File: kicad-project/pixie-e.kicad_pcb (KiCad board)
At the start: 2 copper layers, 55 x 50 mm, 54 parts, among them J1 PWR, J2 ANT, J3 SP, J4 KEY, Q1 2N2222, Q2 2N2222, Q3 2N2222, Q4 2N3906, Q5 2N7000, SW1 PWR, SW2 SW, U1 LM386, U2 STC15W104, U3 LM78L05_TO92, Y1 7.023MHz

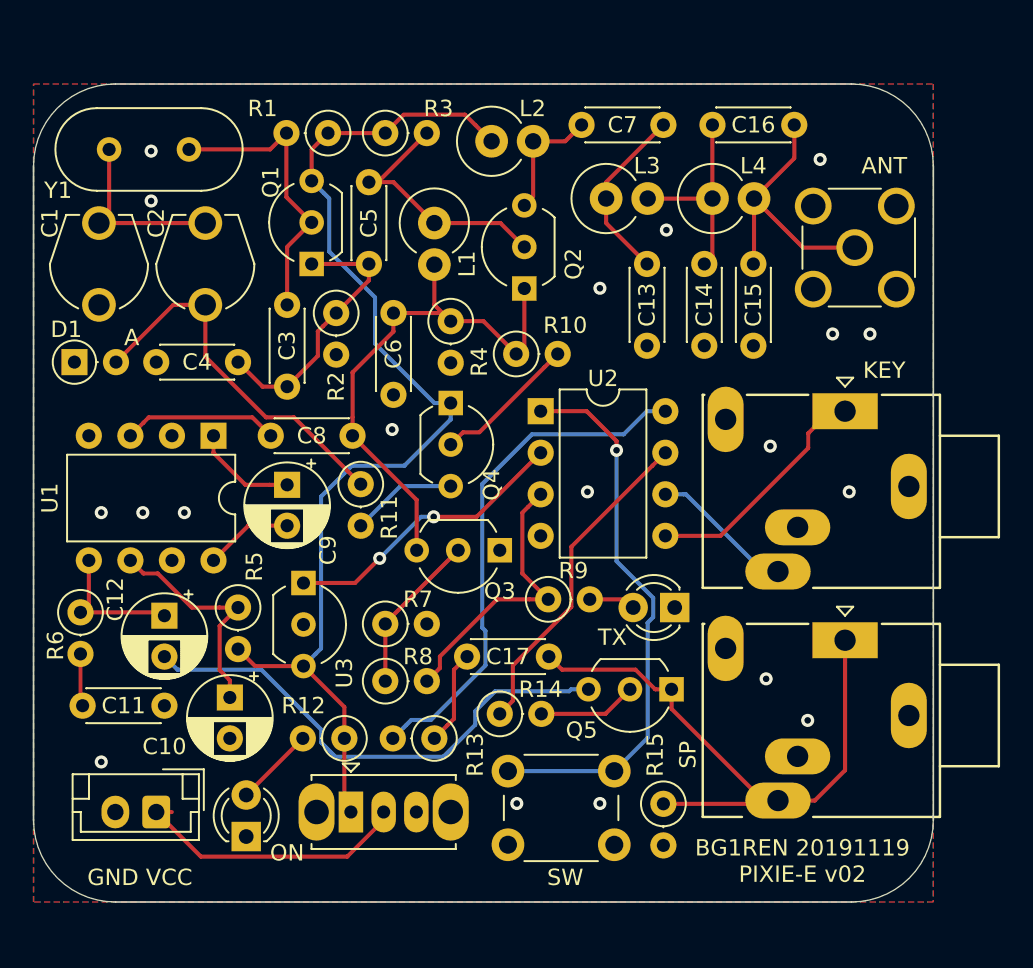
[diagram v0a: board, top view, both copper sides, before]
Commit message: Finish the 1st smt version.
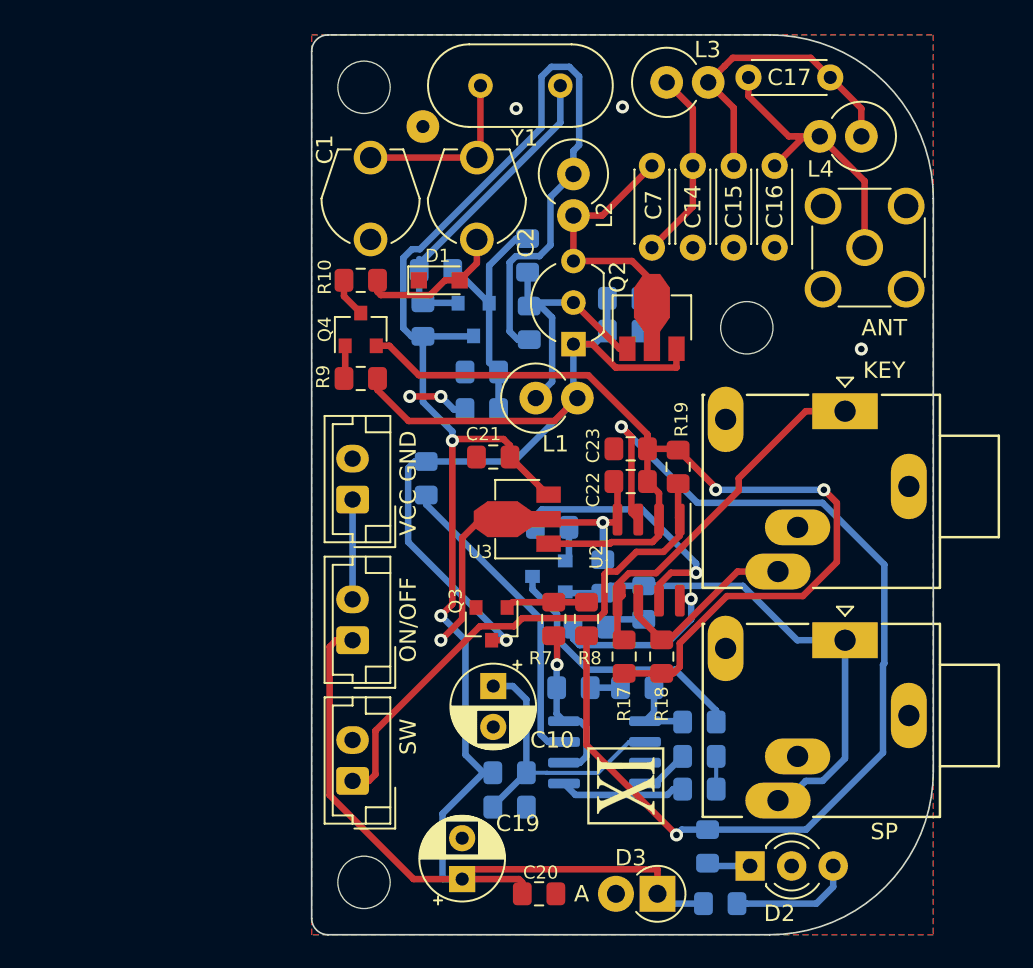
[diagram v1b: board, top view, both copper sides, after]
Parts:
- added C11: 100n, Capacitor_SMD:C_0805_2012Metric_Pad1.15x1.40mm_HandSolder, B.Cu at (129.1, 94.2)
- added C19: 100u, Capacitor_THT:CP_Radial_D5.0mm_P2.50mm, F.Cu at (126.2, 98.6)
- added C20: 100n, Capacitor_SMD:C_0805_2012Metric_Pad1.15x1.40mm_HandSolder, F.Cu at (130.9, 99.5)
- added C21: 330n, Capacitor_SMD:C_0805_2012Metric_Pad1.15x1.40mm_HandSolder, F.Cu at (128.1, 72.8)
- added C22: 100n, Capacitor_SMD:C_0805_2012Metric_Pad1.15x1.40mm_HandSolder, F.Cu at (136.5, 74.3)
- added C23: 10u, Capacitor_SMD:C_0805_2012Metric_Pad1.15x1.40mm_HandSolder, F.Cu at (136.5, 72.3)
- added G***: LOGO, xi:xi-logo-a-07_07, B.Cu at (124.3, 79.6)
- added G***: LOGO, xi:xi-logo-c-05_05, F.Cu at (136.2, 92.9)
- added R16: 1K, Resistor_SMD:R_0805_2012Metric_Pad1.15x1.40mm_HandSolder, B.Cu at (140.7, 93.1)
- added R17: 10K, Resistor_SMD:R_0805_2012Metric_Pad1.15x1.40mm_HandSolder, F.Cu at (136.1, 85.0)
- added R18: 10K, Resistor_SMD:R_0805_2012Metric_Pad1.15x1.40mm_HandSolder, F.Cu at (138.4, 85.0)
- added R19: 10K, Resistor_SMD:R_0805_2012Metric_Pad1.15x1.40mm_HandSolder, F.Cu at (139.4, 73.4)
- added REF**: SOT-89-3, Package_TO_SOT_SMD:SOT-89-3, F.Cu at (137.8, 64.7)
- added REF**: FreeSolderWirePad_1x01_Drill0.8mm, bg1ren:FreeSolderWirePad_1x01_Drill0.8mm, F.Cu at (123.8, 52.6)
- added REF**: MountingHole_3.2mm_M3_DIN965, MountingHole:MountingHole_3.2mm_M3_DIN965, F.Cu at (120.2, 98.8)
- added REF**: MountingHole_3.2mm_M3_DIN965, MountingHole:MountingHole_3.2mm_M3_DIN965, F.Cu at (120.2, 50.2)
- added REF**: MountingHole_3.2mm_M3_DIN965, MountingHole:MountingHole_3.2mm_M3_DIN965, F.Cu at (143.6, 64.9)
- C12: renamed from C11; footprint Capacitor_THT:C_Disc_D4.3mm_W1.9mm_P5.00mm -> Capacitor_SMD:C_0805_2012Metric_Pad1.15x1.40mm_HandSolder; moved to B.Cu
- C13: renamed from C12; footprint Capacitor_THT:CP_Radial_D5.0mm_P2.50mm -> Capacitor_SMD:C_0805_2012Metric_Pad1.15x1.40mm_HandSolder; moved to B.Cu
- C18: renamed from C17; footprint Capacitor_THT:C_Disc_D4.3mm_W1.9mm_P5.00mm -> Capacitor_SMD:C_0805_2012Metric_Pad1.15x1.40mm_HandSolder; moved to B.Cu
- C3, C4, C5, C6, C8: footprint Capacitor_THT:C_Disc_D4.3mm_W1.9mm_P5.00mm -> Capacitor_SMD:C_0805_2012Metric_Pad1.15x1.40mm_HandSolder; moved to B.Cu
- C7: value 10n -> 100n
- C9: footprint Capacitor_THT:CP_Radial_D5.0mm_P2.50mm -> Capacitor_SMD:C_0805_2012Metric_Pad1.15x1.40mm_HandSolder; moved to B.Cu
- D1: footprint Diode_THT:D_DO-35_SOD27_P2.54mm_Vertical_AnodeUp -> Diode_SMD:D_SOD-323_HandSoldering
- D2: value RED -> LED_Dual_ACA; footprint LED_THT:LED_D3.0mm -> LED_THT:LED_D3.0mm-3
- D3: value YELLO -> 1N4001; footprint LED_THT:LED_D3.0mm -> Diode_THT:D_DO-41_SOD81_P2.54mm_Vertical_AnodeUp
- Q1: footprint Package_TO_SOT_THT:TO-92_Inline_Wide -> Package_TO_SOT_SMD:SOT-23; moved to B.Cu
- Q3, Q4: footprint Package_TO_SOT_THT:TO-92_Inline_Wide -> Package_TO_SOT_SMD:SOT-23
- Q5: value 2N7000 -> 2N7002; footprint Package_TO_SOT_THT:TO-92_Inline_Wide -> Package_TO_SOT_SMD:SOT-23; moved to B.Cu
- R1, R13, R14, R15, R3, R4, R6: footprint Resistor_THT:R_Axial_DIN0207_L6.3mm_D2.5mm_P2.54mm_Vertical -> Resistor_SMD:R_0805_2012Metric_Pad1.15x1.40mm_HandSolder; moved to B.Cu
- R10: renamed from R11; value 4.7K -> 1K; footprint Resistor_THT:R_Axial_DIN0207_L6.3mm_D2.5mm_P2.54mm_Vertical -> Resistor_SMD:R_0805_2012Metric_Pad1.15x1.40mm_HandSolder
- R11: renamed from R12; footprint Resistor_THT:R_Axial_DIN0207_L6.3mm_D2.5mm_P2.54mm_Vertical -> Resistor_SMD:R_0805_2012Metric_Pad1.15x1.40mm_HandSolder; moved to B.Cu
- R12: renamed from R9; footprint Resistor_THT:R_Axial_DIN0207_L6.3mm_D2.5mm_P2.54mm_Vertical -> Resistor_SMD:R_0805_2012Metric_Pad1.15x1.40mm_HandSolder; moved to B.Cu
- R2: value 470 -> 1K; footprint Resistor_THT:R_Axial_DIN0207_L6.3mm_D2.5mm_P2.54mm_Vertical -> Resistor_SMD:R_0805_2012Metric_Pad1.15x1.40mm_HandSolder; moved to B.Cu
- R5: value 1K -> 10; footprint Resistor_THT:R_Axial_DIN0207_L6.3mm_D2.5mm_P2.54mm_Vertical -> Resistor_SMD:R_0805_2012Metric_Pad1.15x1.40mm_HandSolder; moved to B.Cu
- R7, R8: footprint Resistor_THT:R_Axial_DIN0207_L6.3mm_D2.5mm_P2.54mm_Vertical -> Resistor_SMD:R_0805_2012Metric_Pad1.15x1.40mm_HandSolder
- R9: renamed from R10; footprint Resistor_THT:R_Axial_DIN0207_L6.3mm_D2.5mm_P2.54mm_Vertical -> Resistor_SMD:R_0805_2012Metric_Pad1.15x1.40mm_HandSolder
- SW1: value PWR -> ON/OFF; footprint Button_Switch_THT:SW_Slide_1P2T_CK_OS102011MS2Q -> Connector_JST:JST_EH_B2B-EH-A_1x02_P2.50mm_Vertical
- SW2: footprint Button_Switch_THT:SW_PUSH_6mm -> Connector_JST:JST_EH_B2B-EH-A_1x02_P2.50mm_Vertical
- U1: footprint Package_DIP:DIP-8_W7.62mm -> Package_SO:SOIC-8_3.9x4.9mm_P1.27mm; moved to B.Cu
- U2: footprint Package_DIP:DIP-8_W7.62mm -> Package_SO:SOIC-8_3.9x4.9mm_P1.27mm
- U3: footprint Package_TO_SOT_THT:TO-92_Inline_Wide -> Package_TO_SOT_SMD:SOT-89-3
- Y1: footprint Crystal:Crystal_HC49-4H_Vertical -> Crystal:Crystal_HC49-U_Vertical
- moved R6 34.3 mm to (136.9, 86.9), turned to 180 degrees
- moved C13 33.3 mm to (140.7, 89.0), turned to 0 degrees
- moved U1 30.8 mm to (134.9, 90.8), turned to 0 degrees
- moved C9 30.2 mm to (140.7, 91.1), turned to 180 degrees
- moved D3 25.4 mm to (138.1, 99.5), turned to 180 degrees
- moved R11 25.1 mm to (142.0, 100.1)
- moved C12 25.0 mm to (133.0, 86.9), turned to 0 degrees
- moved Y1 23.0 mm to (132.2, 50.1)
- moved D1 22.9 mm to (124.8, 62.0)
- moved J1 22.6 mm to (119.5, 75.4), turned to 90 degrees
- moved R5 19.4 mm to (129.1, 92.1), turned to 180 degrees
- moved R12 18.0 mm to (141.2, 96.6), turned to 270 degrees
- moved C1 17.1 mm to (120.6, 57.0)
- moved C2 17.1 mm to (127.1, 57.0)
- moved D2 16.5 mm to (143.8, 97.8), turned to 0 degrees
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- renumbered C13 to C14, C14 to C15, C15 to C16, C16 to C17
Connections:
- net Net-(R8-Pad2) renamed TX-LED
- D2 pad 1: GND -> Net-(D2-Pad1)
- D2 pad 2: Net-(D2-Pad2) -> GND
- D3 pad 1: GND -> VCC
- D3 pad 2: Net-(D3-Pad2) -> GND
- Q1 pad 1: Net-(C3-Pad2) -> Net-(C3-Pad1)
- Q1 pad 2: Net-(C3-Pad1) -> Net-(C3-Pad2)
- Q3 pad 1: GND -> Net-(Q3-Pad1)
- Q3 pad 2: Net-(Q3-Pad2) -> GND
- Q4 pad 1: VCC -> Net-(Q4-Pad1)
- Q4 pad 2: Net-(Q4-Pad2) -> 5V
- Q5 pad 1: Phone -> Net-(Q5-Pad1)
- Q5 pad 2: Net-(Q5-Pad2) -> Phone
- R11 pad 1: VCC -> Net-(D2-Pad3)
- R11 pad 2: Net-(D3-Pad2) -> VCC
- R12 pad 2: Net-(D2-Pad2) -> Net-(D2-Pad1)
- R14 pad 2: Net-(Q5-Pad2) -> Net-(Q5-Pad1)
- R7 pad 1: Net-(Q3-Pad2) -> Net-(Q3-Pad1)
- R8 pad 1: Net-(Q3-Pad2) -> Net-(Q3-Pad1)
- R9 pad 2: Net-(Q4-Pad2) -> Net-(Q4-Pad1)
- U1 pad 1: Net-(C9-Pad1) -> Net-(R16-Pad2)
- U1 pad 7: Net-(U1-Pad7) -> (no net)
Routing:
- net VCC: track 68.4 -> 134.9 mm, vias 0 -> 2
- net TX-LED: track 17.4 -> 66.4 mm, vias 0 -> 2
- net 5V: track 17.8 -> 65.6 mm
- net GND: track 0.00 -> 33.5 mm, vias 19 -> 8
- net KEY: track 33.8 -> 56.2 mm, vias 0 -> 1
- net Sidetone: track 31.7 -> 10.7 mm, vias 0 -> 1
- net AF: track 31.1 -> 16.7 mm
- net SHIFT: track 22.8 -> 9.12 mm
- net Net-(J1-Pad1): track 17.4 -> 6.10 mm
- net Net-(C7-Pad2): track 7.52 -> 18.1 mm
- net DIT: track 14.7 -> 25.0 mm
- net Net-(Q3-Pad2): track 9.85 -> 0.00 mm
- net Net-(C8-Pad2): track 9.51 -> 19.2 mm
- net Net-(Q4-Pad2): track 8.83 -> 0.00 mm
- net Net-(R16-Pad2): track 0.00 -> 7.69 mm
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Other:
- board size 55 x 50 mm -> 38 x 55 mm
- board text added: "JLCJLCJLCJLC"
- board text added: "PIXIE-E v03s, BG1REN 20200111"
- board text added: "VCC GND"
- board text removed: "BG1REN 20191119 PIXIE-E v02"
- board text removed: "GND VCC"
